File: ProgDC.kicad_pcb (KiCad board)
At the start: 2 copper layers, 145 x 100 mm, 51 parts, among them J1 Conn_02x20_Counter_Clockwise_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, J2 Conn_01x24_Pin, J3 Conn_01x03_Pin, U1 KR580VK28, U2 628512, U3 CPU

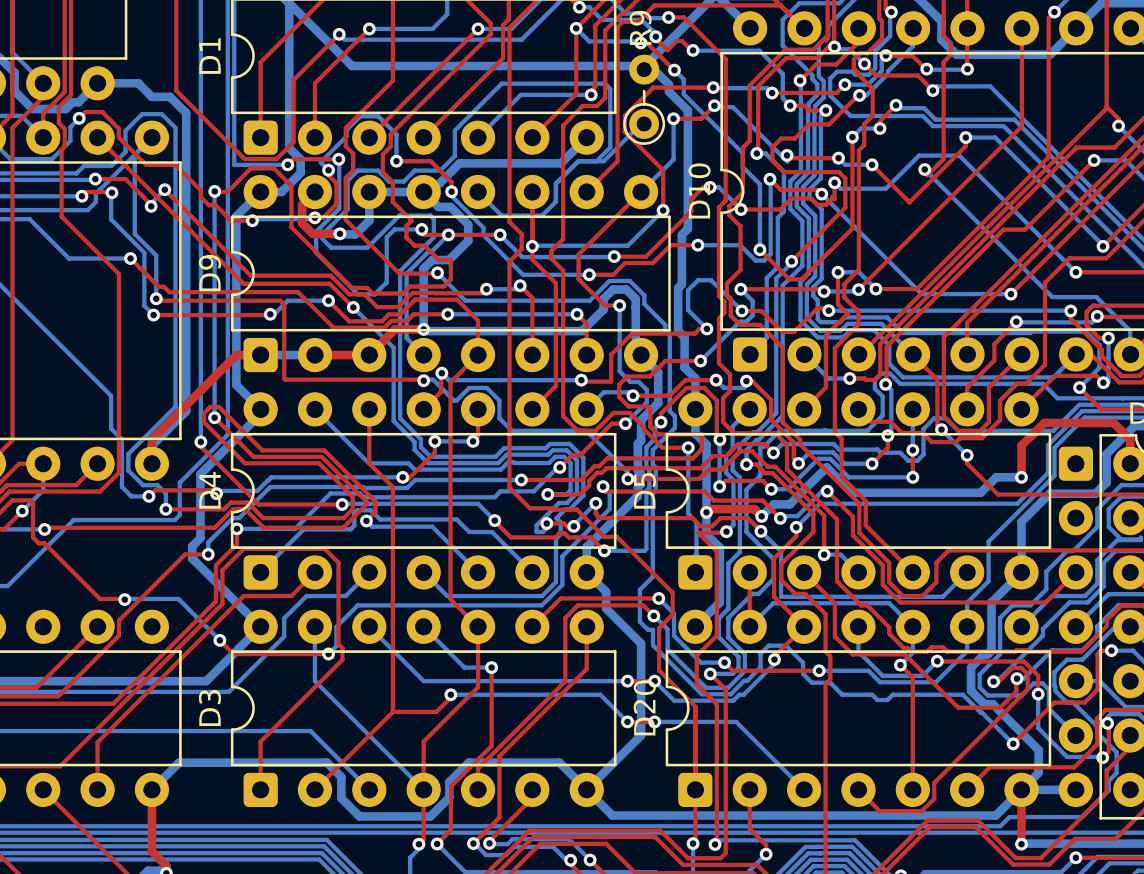
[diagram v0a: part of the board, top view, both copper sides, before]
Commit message: Fix bugs
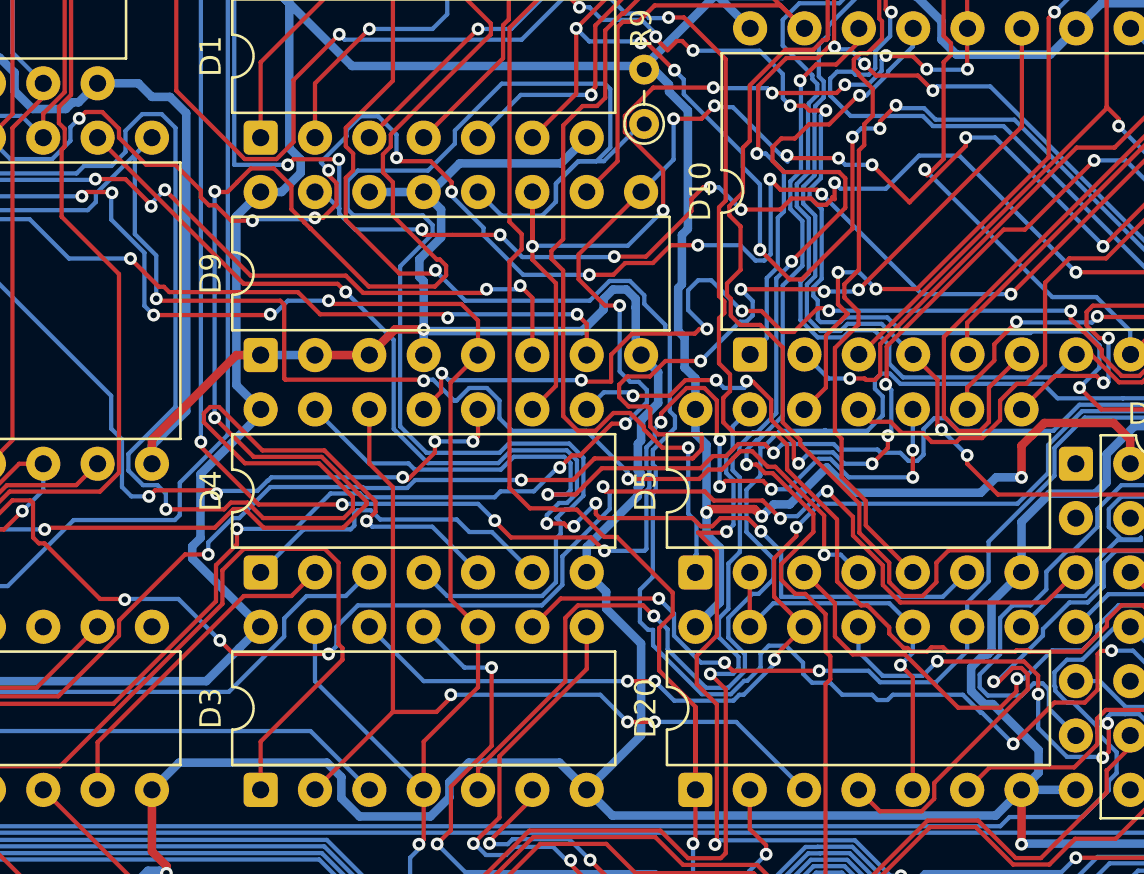
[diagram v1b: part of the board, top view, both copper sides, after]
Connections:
- net Net-(D2.1-B) renamed /~{A_FF}
- D9 pad 15: GND -> Net-(D14.3-Y)
- D9 pad 4: Net-(D14.3-Y) -> GND
- R8 pad 1: Net-(D23.1-~{R}) -> unconnected-(R8-Pad1)
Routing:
- net Net-(D14.3-Y): track 123.6 -> 111.7 mm, vias 11 -> 10
- net GND: track 623.0 -> 615.3 mm, vias 11 -> 10
- net /P0: track 75.4 -> 70.5 mm
- net /AB6: track 345.8 -> 343.9 mm
- net /~{RESET}: track 60.7 -> 59.7 mm
- net /Q7: track 234.6 -> 233.7 mm
- net /Q6: track 56.0 -> 55.4 mm
